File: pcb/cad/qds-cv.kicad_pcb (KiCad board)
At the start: 4 copper layers, 219 x 159 mm, 114 parts, among them J201 Conn_Coaxial, J701 Conn_Coaxial, J702 DB9_Female, K701 FINDER-30.22, Q701 BC846B, SW601 SW_DIP_x05, SW701 RST, SW702 TRIG, U201 OPA2227, U202 AMC1200, U203 AD8421, U204 LM393-N, U601 74HC32D, U602 74HC123, U603 74HCS08, U701 74HCS08, U702 74HC574, U703 74LV132, U704 74LVC2G17, U705 74LVC2G17, U706 HFBR-1521Z, U801 OPA2227, U802 MAX6350CSA

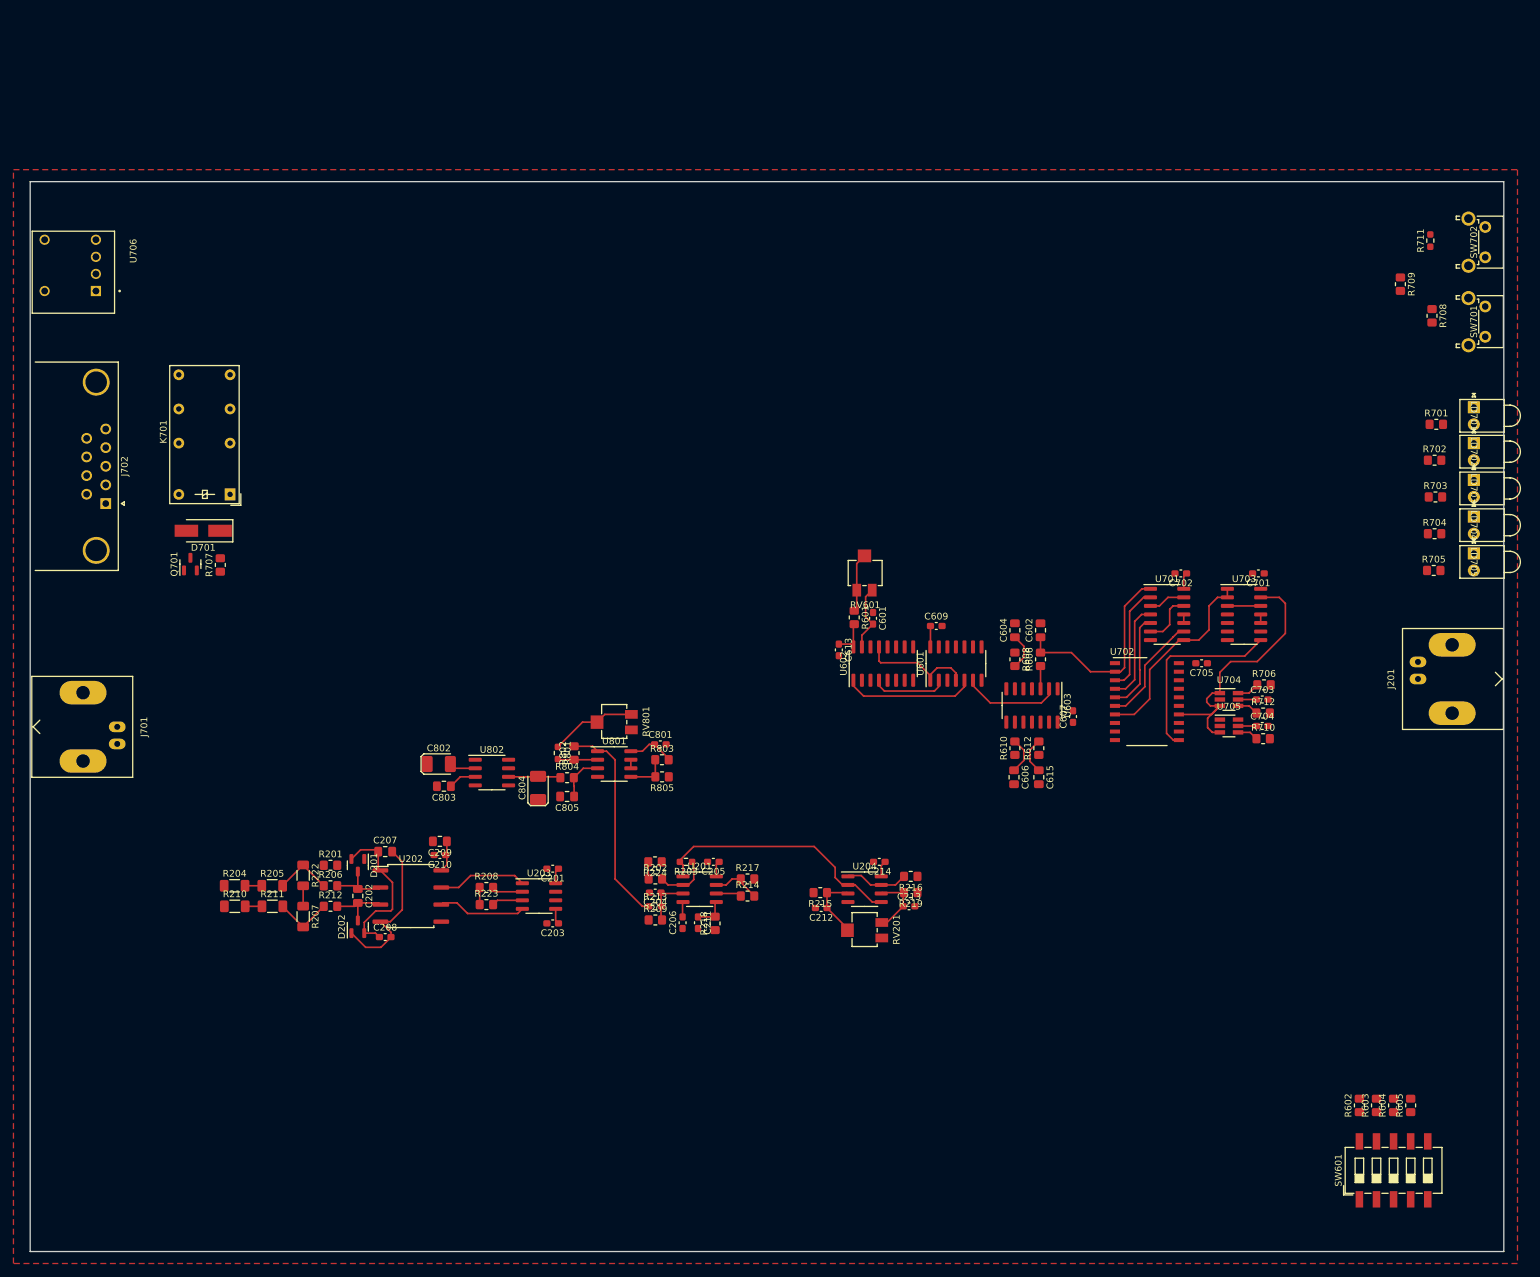
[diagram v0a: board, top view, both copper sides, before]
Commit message: Include ISO-A power circuit, all connectors and test points on PCB
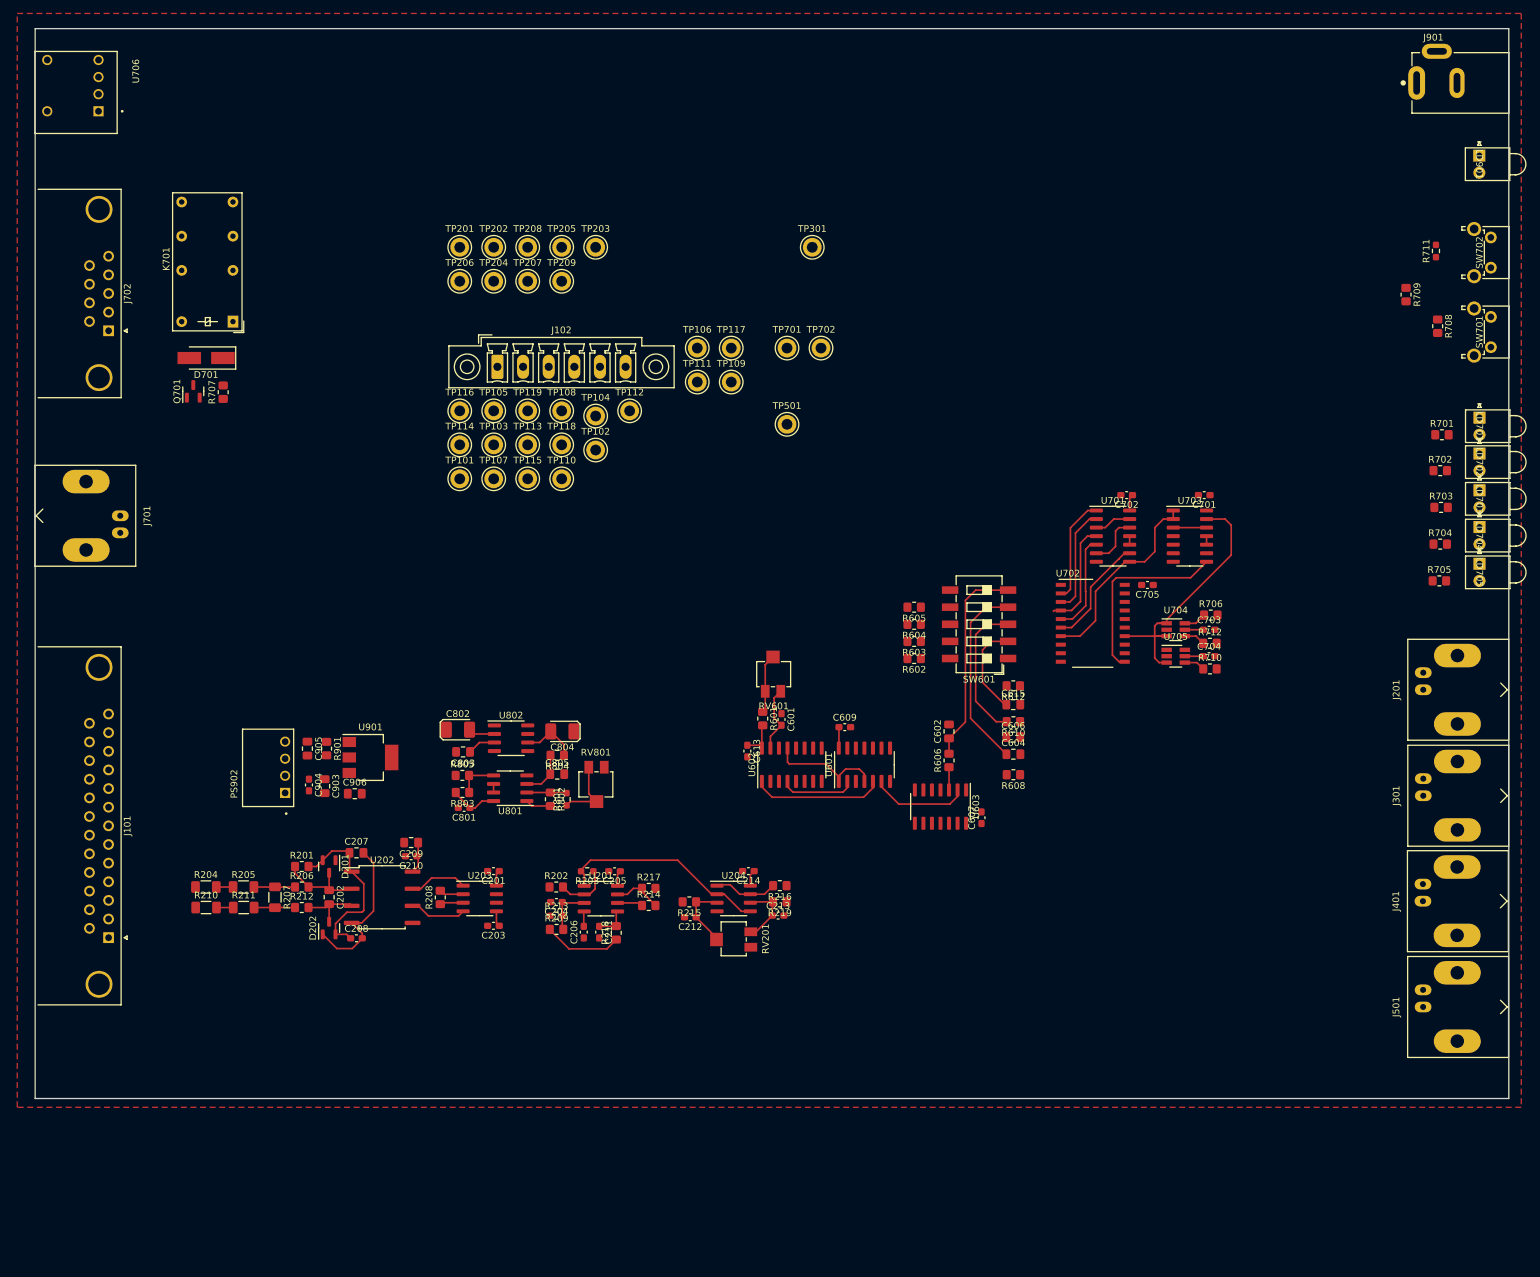
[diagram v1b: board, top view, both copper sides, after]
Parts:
- removed R222: 0, Resistor_SMD:R_1206_3216Metric_Pad1.30x1.75mm_HandSolder
- removed R223, R224: 0, Resistor_SMD:R_0805_2012Metric_Pad1.20x1.40mm_HandSolder
- added C903: 10u, Capacitor_SMD:C_0805_2012Metric_Pad1.18x1.45mm_HandSolder, F.Cu at (143.0, 152.6)
- added C904: 100n, Capacitor_SMD:C_0603_1608Metric_Pad1.08x0.95mm_HandSolder, F.Cu at (140.7, 152.4)
- added C905: 10u, Capacitor_SMD:C_0805_2012Metric_Pad1.18x1.45mm_HandSolder, F.Cu at (140.5, 147.0)
- added C906: 10u, Capacitor_SMD:C_0805_2012Metric_Pad1.18x1.45mm_HandSolder, F.Cu at (147.5, 153.7)
- added J101: DB25 Female, Connector_Dsub:DSUB-25_Female_Horizontal_P2.77x2.84mm_EdgePinOffset7.70mm_Housed_MountingHolesOffset9.12mm, F.Cu at (110.9, 175.1)
- added J102: Conn_01x08, Connector_Phoenix_MC:PhoenixContact_MCV_1,5_6-GF-3.81_1x06_P3.81mm_Vertical_ThreadedFlange, F.Cu at (168.7, 90.3)
- added J301: Conn_Coaxial, qds-cv-lib:Molex_0731375003, F.Cu at (306.3, 154.0)
- added J401: Conn_Coaxial, qds-cv-lib:Molex_0731375003, F.Cu at (306.2, 169.7)
- added J501: Conn_Coaxial, qds-cv-lib:Molex_0731375003, F.Cu at (306.3, 185.4)
- added J901: Barrel_Jack_Switch, qds-cv-lib:CUI_PJ-002AH, F.Cu at (305.3, 48.1)
- added LD901: Green, qds-cv-lib:LED_WP934CB_GD, F.Cu at (314.6, 58.9)
- added PS902: RI-1515S/P, qds-cv-lib:RI-1515S, F.Cu at (134.6, 149.9)
- added R901: 1.3k, Resistor_SMD:R_0805_2012Metric_Pad1.20x1.40mm_HandSolder, F.Cu at (143.3, 147.0)
- added TP101: VT1, qds-cv-lib:TestPoint_Keystone_5010-5014_Multipurpose, F.Cu at (163.1, 106.9)
- added TP102: VT2, qds-cv-lib:TestPoint_Keystone_5010-5014_Multipurpose, F.Cu at (183.3, 102.6)
- added TP103: TestPoint, qds-cv-lib:TestPoint_Keystone_5010-5014_Multipurpose, F.Cu at (168.1, 101.9)
- added TP104: TestPoint, qds-cv-lib:TestPoint_Keystone_5010-5014_Multipurpose, F.Cu at (183.3, 97.6)
- added TP105: TestPoint, qds-cv-lib:TestPoint_Keystone_5010-5014_Multipurpose, F.Cu at (168.1, 96.8)
- added TP106: TestPoint, qds-cv-lib:TestPoint_Keystone_5010-5014_Multipurpose, F.Cu at (198.4, 87.5)
- added TP107: TestPoint, qds-cv-lib:TestPoint_Keystone_5010-5014_Multipurpose, F.Cu at (168.1, 106.9)
- added TP108: TestPoint, qds-cv-lib:TestPoint_Keystone_5010-5014_Multipurpose, F.Cu at (178.2, 96.8)
- added TP109: TestPoint, qds-cv-lib:TestPoint_Keystone_5010-5014_Multipurpose, F.Cu at (203.4, 92.5)
- added TP110: TestPoint, qds-cv-lib:TestPoint_Keystone_5010-5014_Multipurpose, F.Cu at (178.2, 106.9)
- added TP111: TestPoint, qds-cv-lib:TestPoint_Keystone_5010-5014_Multipurpose, F.Cu at (198.4, 92.5)
- added TP112: TestPoint, qds-cv-lib:TestPoint_Keystone_5010-5014_Multipurpose, F.Cu at (188.3, 96.8)
- added TP113: TestPoint, qds-cv-lib:TestPoint_Keystone_5010-5014_Multipurpose, F.Cu at (173.2, 101.9)
- added TP114: TestPoint, qds-cv-lib:TestPoint_Keystone_5010-5014_Multipurpose, F.Cu at (163.1, 101.9)
- added TP115: TestPoint, qds-cv-lib:TestPoint_Keystone_5010-5014_Multipurpose, F.Cu at (173.2, 106.9)
- added TP116: TestPoint, qds-cv-lib:TestPoint_Keystone_5010-5014_Multipurpose, F.Cu at (163.1, 96.8)
- added TP117: TestPoint, qds-cv-lib:TestPoint_Keystone_5010-5014_Multipurpose, F.Cu at (203.4, 87.5)
- added TP118: TestPoint, qds-cv-lib:TestPoint_Keystone_5010-5014_Multipurpose, F.Cu at (178.2, 101.9)
- added TP119: TestPoint, qds-cv-lib:TestPoint_Keystone_5010-5014_Multipurpose, F.Cu at (173.2, 96.8)
- added TP201: Vth-H, qds-cv-lib:TestPoint_Keystone_5010-5014_Multipurpose, F.Cu at (163.1, 72.5)
- added TP202: Vth-L, qds-cv-lib:TestPoint_Keystone_5010-5014_Multipurpose, F.Cu at (168.1, 72.5)
- added TP203: TestPoint, qds-cv-lib:TestPoint_Keystone_5010-5014_Multipurpose, F.Cu at (183.3, 72.5)
- added TP204: TestPoint, qds-cv-lib:TestPoint_Keystone_5010-5014_Multipurpose, F.Cu at (168.1, 77.5)
- added TP205: TestPoint, qds-cv-lib:TestPoint_Keystone_5010-5014_Multipurpose, F.Cu at (178.2, 72.5)
- added TP206: TestPoint, qds-cv-lib:TestPoint_Keystone_5010-5014_Multipurpose, F.Cu at (163.1, 77.5)
- added TP207: TestPoint, qds-cv-lib:TestPoint_Keystone_5010-5014_Multipurpose, F.Cu at (173.2, 77.5)
- added TP208: TestPoint, qds-cv-lib:TestPoint_Keystone_5010-5014_Multipurpose, F.Cu at (173.2, 72.5)
- added TP209: V-DET, qds-cv-lib:TestPoint_Keystone_5010-5014_Multipurpose, F.Cu at (178.2, 77.5)
- added TP301: RCx, qds-cv-lib:TestPoint_Keystone_5010-5014_Multipurpose, F.Cu at (215.5, 72.5)
- added TP501: 5V-REF, qds-cv-lib:TestPoint_Keystone_5010-5014_Multipurpose, F.Cu at (211.7, 98.8)
- added TP701: TestPoint, qds-cv-lib:TestPoint_Keystone_5010-5014_Multipurpose, F.Cu at (211.7, 87.5)
- added TP702: TestPoint, qds-cv-lib:TestPoint_Keystone_5010-5014_Multipurpose, F.Cu at (216.8, 87.5)
- added U901: LT1129CST-5, Package_TO_SOT_SMD:SOT-223-3_TabPin2, F.Cu at (149.8, 148.3)
- moved R605 104.5 mm to (230.6, 126.0), turned to 180 degrees
- moved SW601 101.9 mm to (240.3, 128.5), turned to 180 degrees
- moved R604 100.9 mm to (230.6, 128.5), turned to 180 degrees
- moved R603 97.3 mm to (230.6, 131.1), turned to 180 degrees
- moved R602 93.8 mm to (230.6, 133.6), turned to 180 degrees
- moved J701 31.4 mm to (112.6, 112.4)
- moved C801 30.7 mm to (163.7, 155.8), turned to 180 degrees
- moved R803 30.0 mm to (163.5, 153.5), turned to 180 degrees
- moved R805 29.7 mm to (163.5, 151.0), turned to 0 degrees
- moved U706 26.7 mm to (101.8, 48.5)
- moved K701 25.7 mm to (129.4, 83.5)
- moved Q701 25.7 mm to (123.5, 93.9)
- moved R707 25.7 mm to (127.9, 94.0)
- moved D701 25.7 mm to (125.4, 89.0)
- moved J702 25.7 mm to (110.9, 84.9)
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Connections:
- R202 pad 1: Net-(R202-Pad1) -> Earth
- R207 pad 1: Net-(R207-Pad1) -> Net-(R205-Pad2)
- R208 pad 1: Net-(R208-Pad1) -> Net-(U203-Pad3)
- SW601 pad 1: /Detection validation/TRIG-CH-A -> unconnected-(SW601-Pad1)
- SW601 pad 10: Net-(R602-Pad1) -> unconnected-(SW601-Pad10)
- SW601 pad 2: /Detection validation/TRIG-CH-B -> /Detection validation/TRIG-CH-D
- SW601 pad 4: /Detection validation/TRIG-CH-D -> /Detection validation/TRIG-CH-B
- SW601 pad 5: unconnected-(SW601-Pad5) -> /Detection validation/TRIG-CH-A
- SW601 pad 6: unconnected-(SW601-Pad6) -> Net-(R602-Pad1)
- SW601 pad 7: Net-(R605-Pad1) -> Net-(R603-Pad1)
- SW601 pad 9: Net-(R603-Pad1) -> Net-(R605-Pad1)
- U203 pad 3: Net-(R223-Pad2) -> Net-(U203-Pad3)
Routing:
- net /+5V reference/+5VREF: track 31.4 -> 3.80 mm
- net /Detection validation/TRIG-CH-B: track 21.3 -> 44.2 mm
- net /Detection validation/TRIG-CH-C: track 20.4 -> 37.3 mm
- net /Detection validation/TRIG-CH-A: track 30.3 -> 46.5 mm
- net Net-(R209-Pad1): track 0.00 -> 11.7 mm
- net /Detection validation/TRIG-CH-D: track 20.2 -> 28.8 mm
- net /Isolated detection channel A/V-DET: track 37.7 -> 31.5 mm
- net Net-(U202-Pad6): track 13.1 -> 8.42 mm
- net Net-(U202-Pad7): track 13.3 -> 8.65 mm
- net Net-(R223-Pad2): track 4.61 -> 0.00 mm
- net Net-(C202-Pad1): track 9.28 -> 13.2 mm
- net Net-(U203-Pad3): track 0.00 -> 3.48 mm
- net Net-(R207-Pad1): track 3.02 -> 0.00 mm
- net Net-(R801-Pad1): track 12.9 -> 10.3 mm
- net Net-(R205-Pad2): track 8.73 -> 6.16 mm
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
